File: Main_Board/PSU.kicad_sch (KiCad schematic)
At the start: 20 parts, among them J3 Baterry input

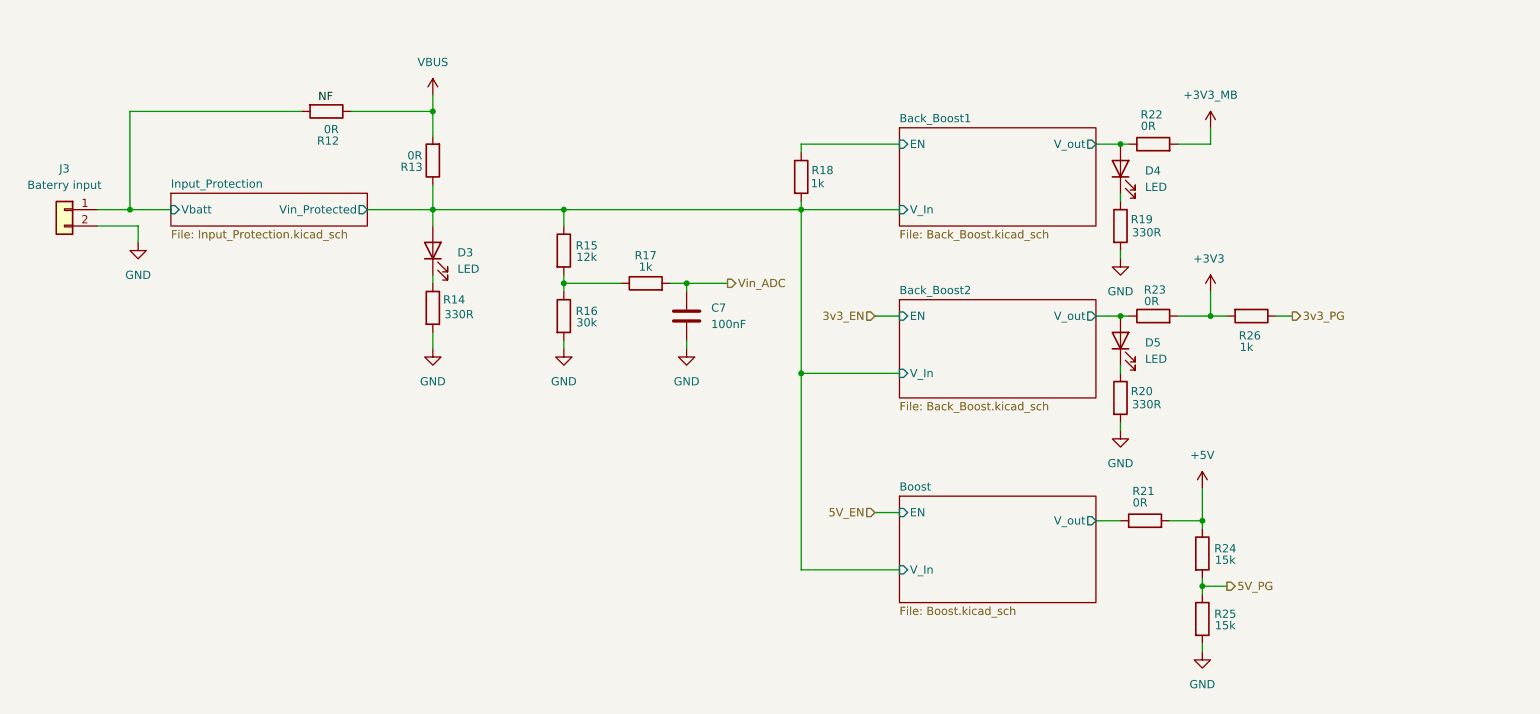
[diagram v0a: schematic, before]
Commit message: Small fix
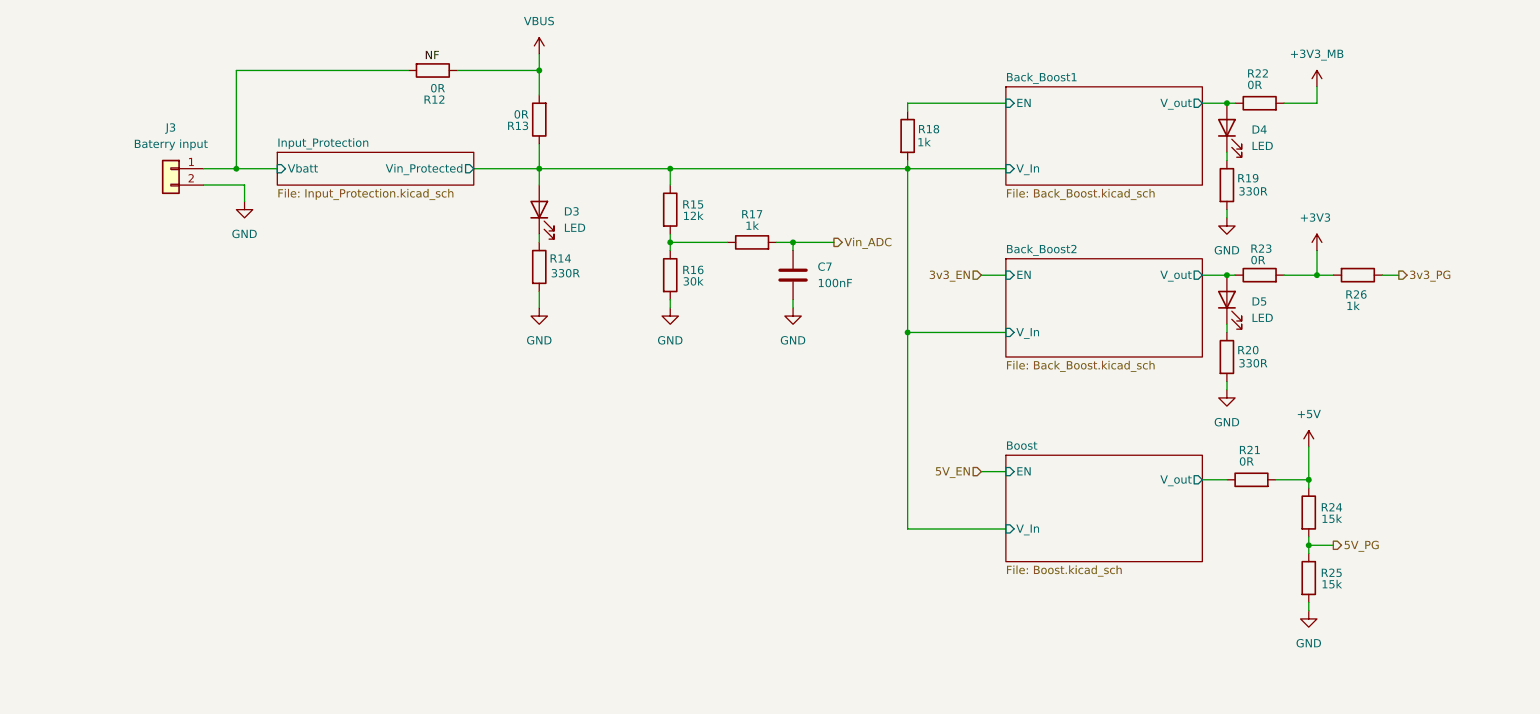
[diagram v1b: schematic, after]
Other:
- moved on the sheet: C7, D3, D4, D5, J3, R12, R13, R14, R15, R16, R17, R18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

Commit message: fix shema after review
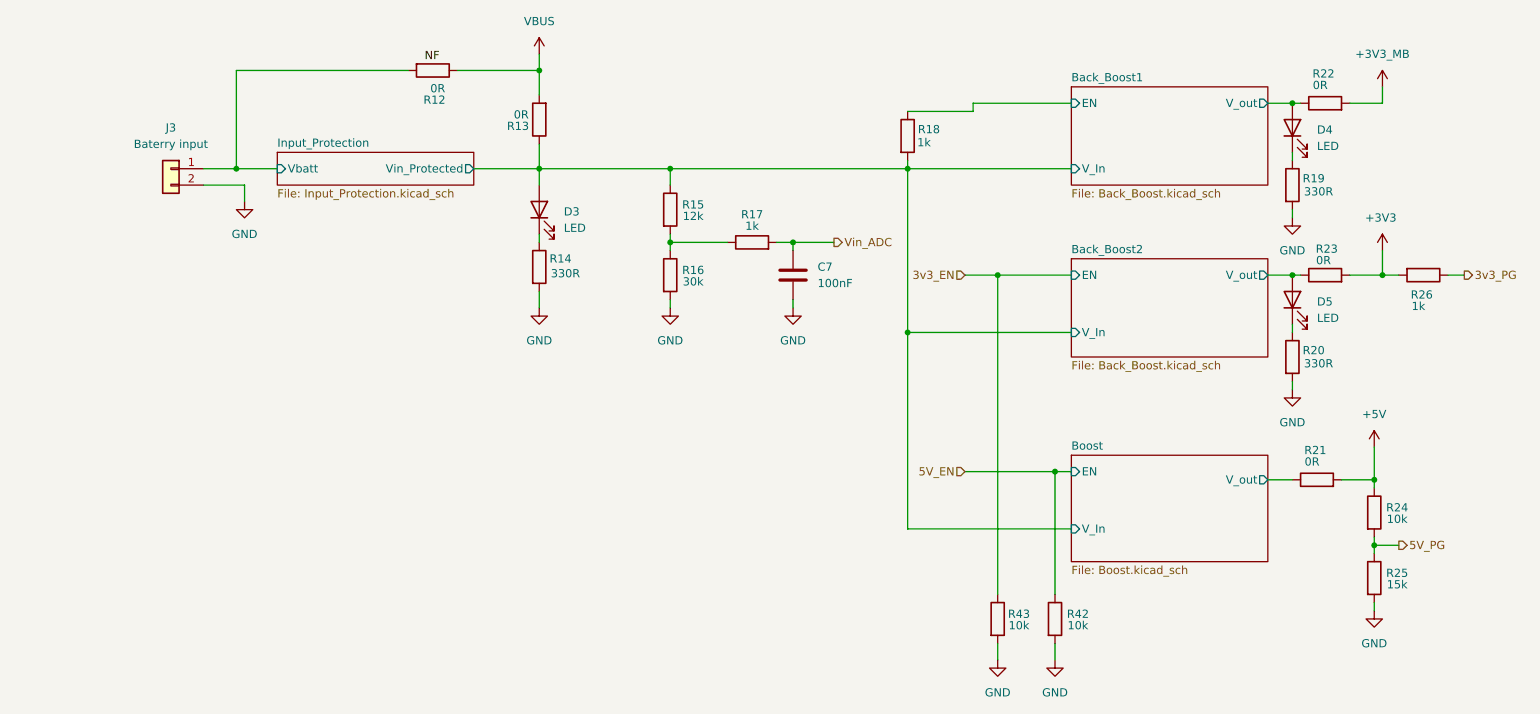
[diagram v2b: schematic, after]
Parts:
- added R42, R43: 10k, Resistor_SMD:R_0603_1608Metric, symbol Device:R
- R24: value 15k -> 10k
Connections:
- net 3v3_EN: now also R43.1
- net 5V_EN: now also R42.1
- net GND: now also R42.2, R43.2
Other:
- moved on the sheet: D4, D5, R19, R20, R21, R22, R23, R24, R25, R26

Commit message: fix after review -?D7/D8 clamp to 3v3 MB not for 3v3 and other fix
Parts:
- R13: footprint Resistor_SMD:R_0603_1608Metric -> Resistor_SMD:R_0805_2012Metric
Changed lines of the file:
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@@
 			)
 		)
-		(property "Footprint" "Resistor_SMD:R_0603_1608Metric"
+		(property "Footprint" "Resistor_SMD:R_0805_2012Metric"
 			(at 104.648 66.04 90)
 			(hide yes)
